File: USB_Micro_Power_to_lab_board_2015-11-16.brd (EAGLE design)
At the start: 16.9 x 20.2 mm, 4 parts

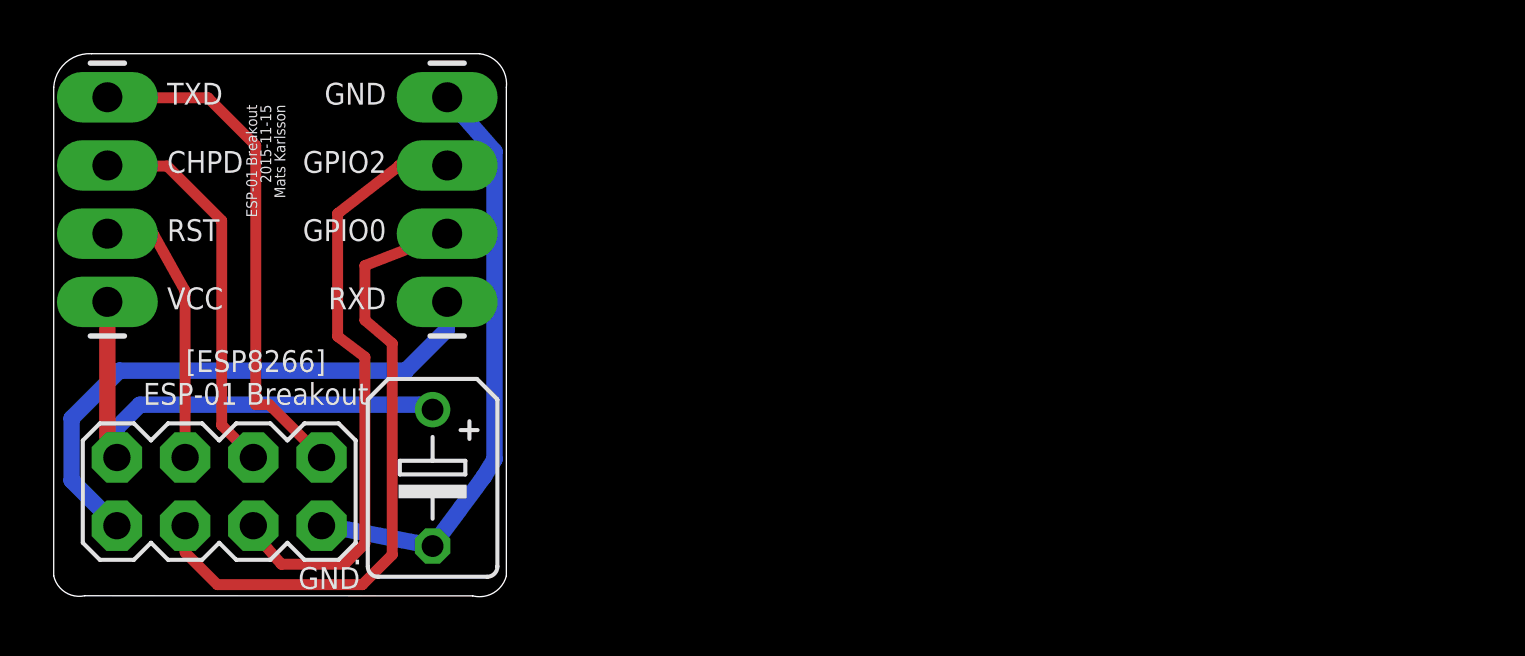
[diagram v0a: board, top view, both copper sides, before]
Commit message: Cleanup
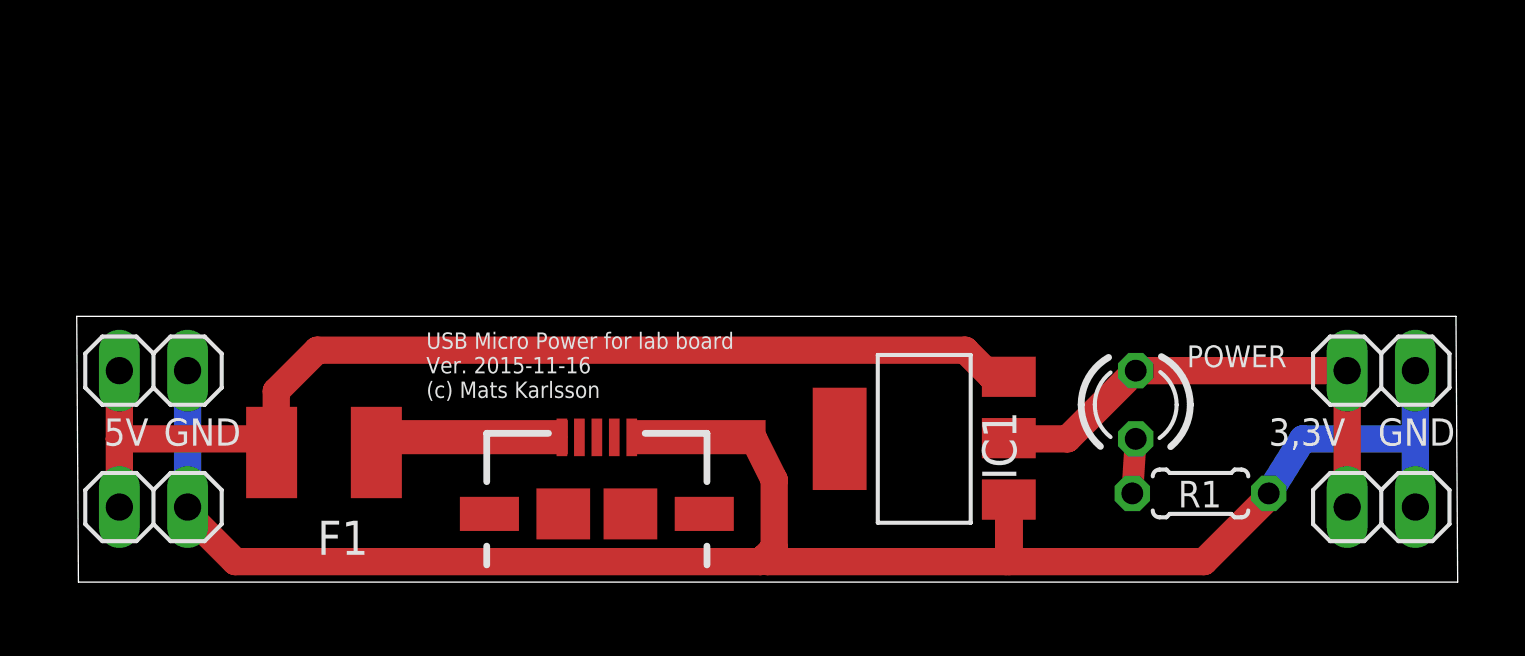
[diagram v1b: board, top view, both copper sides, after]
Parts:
- removed C1: (no value), rcl:B45181B
- removed ESP-01: M04X2, SparkFun-Connectors:2X4
- removed LEFT, RIGHT: (no value), SparkFun-Connectors:1X04_LONGPADS
- added F1: LITTELFUSE_1812_500MA, fuses_polyswitch:R1812
- added IC1: REG1117, burr-brown:SOT223
- added JP1, JP2, JP3, JP4: (no value), pinhead:1X02
- added POWER: (no value), led:LED3MM
- added R1: (no value), resistor:0204/5
- added U1: (no value), Testing:USB-AB-MICRO-SMD_VO2
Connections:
- removed net CH_PD: ESP-01.3, LEFT.2
- removed net GPIO0: ESP-01.6, RIGHT.3
- removed net GPIO2: ESP-01.4, RIGHT.2
- removed net RST: ESP-01.5, LEFT.3
- removed net RXD: ESP-01.8, RIGHT.4
- removed net TXD: ESP-01.1, LEFT.1
- removed net VCC: C1.+, ESP-01.7, LEFT.4
- new net N$1: F1.2, IC1.3, JP1.1, JP3.1
- new net N$2: F1.1, U1.VBUS
- new net N$4: POWER.K, R1.2
- new net N$5: IC1.2, JP2.1, JP4.1, POWER.A
- net GND: now also IC1.1, JP1.2, JP2.2, JP3.2, JP4.2, R1.1, U1.GND; no longer C1.-, ESP-01.2, RIGHT.1
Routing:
- net GND: track 22.3 -> 72.1 mm
- net N$1: track 0.00 -> 41.9 mm
- net GPIO0: track 24.2 -> 0.00 mm
- net GPIO2: track 22.8 -> 0.00 mm
- net RXD: track 21.1 -> 0.00 mm
- net TXD: track 19.2 -> 0.00 mm
- net VCC: track 19.2 -> 0.00 mm
- net N$5: track 0.00 -> 18.8 mm
- net CH_PD: track 14.4 -> 0.00 mm
- net N$2: track 0.00 -> 14.1 mm
- net RST: track 10.3 -> 0.00 mm
- net N$4: track 0.00 -> 2.04 mm
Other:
- board size 16.9 x 20.2 mm -> 51.4 x 9.9 mm
- board text added: "3,3V"
- board text added: "5V"
- board text added: "USB Micro Power for lab board Ver. 2015-11-16 (c) Mats Karlsson"
- board text removed: "."
- board text removed: "CHPD"
- board text removed: "ESP-01 Breakout 2015-11-15 Mats Karlsson"
- board text removed: "GPIO0"
- board text removed: "GPIO2"
- board text removed: "RST"
- board text removed: "RXD"
- board text removed: "TXD"
- board text removed: "VCC"
- board text removed: "[ESP8266] ESP-01 Breakout"

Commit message: Updates
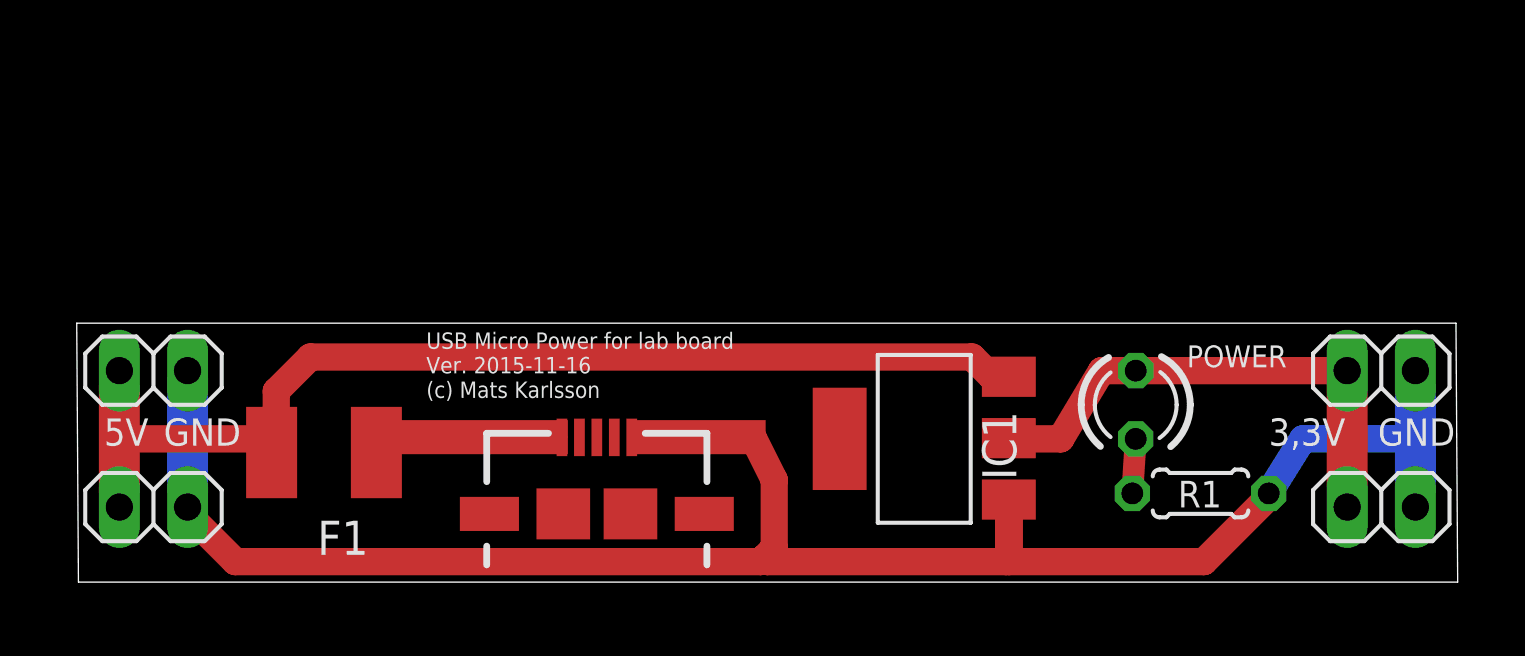
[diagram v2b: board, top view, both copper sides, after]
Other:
- board size 51.4 x 9.9 mm -> 51.4 x 9.6 mm
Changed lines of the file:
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@@
 <plain>
 <wire x1="1.016" y1="-0.254" x2="52.375" y2="-0.254" width="0" layer="20"/>
-<wire x1="52.375" y1="-0.254" x2="52.3115" y2="9.642" width="0" layer="20"/>
-<wire x1="52.3115" y1="9.642" x2="0.9525" y2="9.642" width="0" layer="20"/>
-<wire x1="0.9525" y1="9.642" x2="1.016" y2="-0.254" width="0" layer="20"/>
+<wire x1="52.375" y1="-0.254" x2="52.3115" y2="9.388" width="0" layer="20"/>
+<wire x1="52.3115" y1="9.388" x2="0.9525" y2="9.388" width="0" layer="20"/>
+<wire x1="0.9525" y1="9.388" x2="1.016" y2="-0.254" width="0" layer="20"/>
 <text x="4.191" y="4.826" size="1.016" layer="25" font="vector" ratio="12">GND</text>
 <text x="1.9685" y="4.826" size="1.016" layer="25" font="vector" ratio="12">5V</text>
@@
 Ver. 2015-11-16
 (c) Mats Karlsson</text>
+<rectangle x1="4.318" y1="3.048" x2="5.842" y2="7.366" layer="16"/>
+<rectangle x1="50.038" y1="3.048" x2="51.562" y2="7.112" layer="16"/>
+<rectangle x1="1.778" y1="3.048" x2="3.302" y2="7.112" layer="1"/>
+<rectangle x1="47.498" y1="3.302" x2="49.022" y2="7.112" layer="1"/>
 </plain>
 <attributes>
@@
 <contactref element="JP3" pad="1"/>
 <wire x1="35.6616" y1="7.3914" x2="35.0266" y2="7.3914" width="1.016" layer="1"/>
-<wire x1="35.0266" y1="7.3914" x2="34.036" y2="8.382" width="1.016" layer="1"/>
-<wire x1="34.036" y1="8.382" x2="9.906" y2="8.382" width="1.016" layer="1"/>
-<wire x1="9.906" y1="8.382" x2="8.382" y2="6.858" width="1.016" layer="1"/>
+<wire x1="35.0266" y1="7.3914" x2="34.29" y2="8.128" width="1.016" layer="1"/>
+<wire x1="34.29" y1="8.128" x2="9.652" y2="8.128" width="1.016" layer="1"/>
+<wire x1="9.652" y1="8.128" x2="8.382" y2="6.858" width="1.016" layer="1"/>
 <wire x1="8.382" y1="6.858" x2="8.382" y2="4.744" width="1.016" layer="1"/>
 <wire x1="8.382" y1="4.744" x2="8.21" y2="4.572" width="1.016" layer="1"/>
@@
 <wire x1="48.26" y1="7.62" x2="48.26" y2="2.54" width="1.016" layer="1"/>
 <wire x1="35.6616" y1="5.1054" x2="35.6616" y2="5.08" width="1.016" layer="1"/>
-<wire x1="35.6616" y1="5.08" x2="37.846" y2="5.08" width="1.016" layer="1"/>
-<wire x1="37.846" y1="5.08" x2="40.386" y2="7.62" width="1.016" layer="1"/>
+<wire x1="35.6616" y1="5.08" x2="37.592" y2="5.08" width="1.016" layer="1"/>
+<wire x1="37.592" y1="5.08" x2="39.116" y2="7.62" width="1.016" layer="1"/>
+<wire x1="39.116" y1="7.62" x2="40.386" y2="7.62" width="1.016" layer="1"/>
 <wire x1="40.386" y1="7.62" x2="48.26" y2="7.62" width="1.016" layer="1"/>
 </signal>
